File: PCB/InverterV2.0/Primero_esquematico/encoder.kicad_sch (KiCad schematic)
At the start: 25 parts, among them J5 348250125, U31 TPD4E05U06DQA, U32 TPD4E05U06DQA, U35 SN65HVD82DR, U36 AM26LS32AIDR, U37 SN74LVC245ANSR, U38 TPD4E05U06DQA

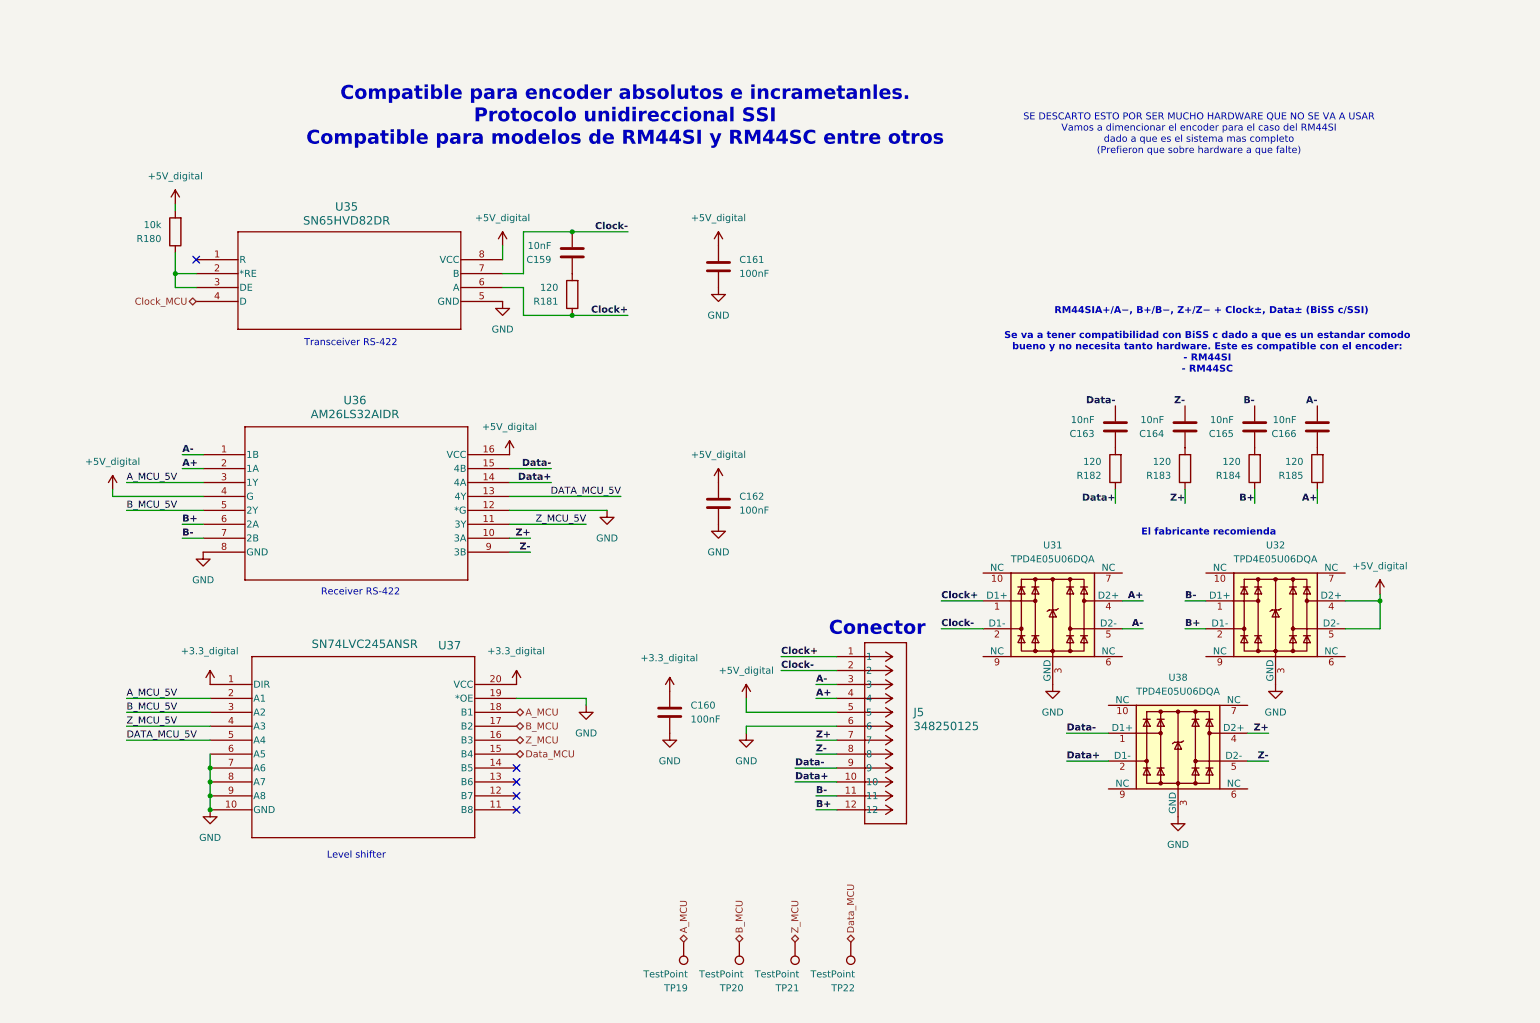
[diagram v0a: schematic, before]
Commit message: aislacion encoder
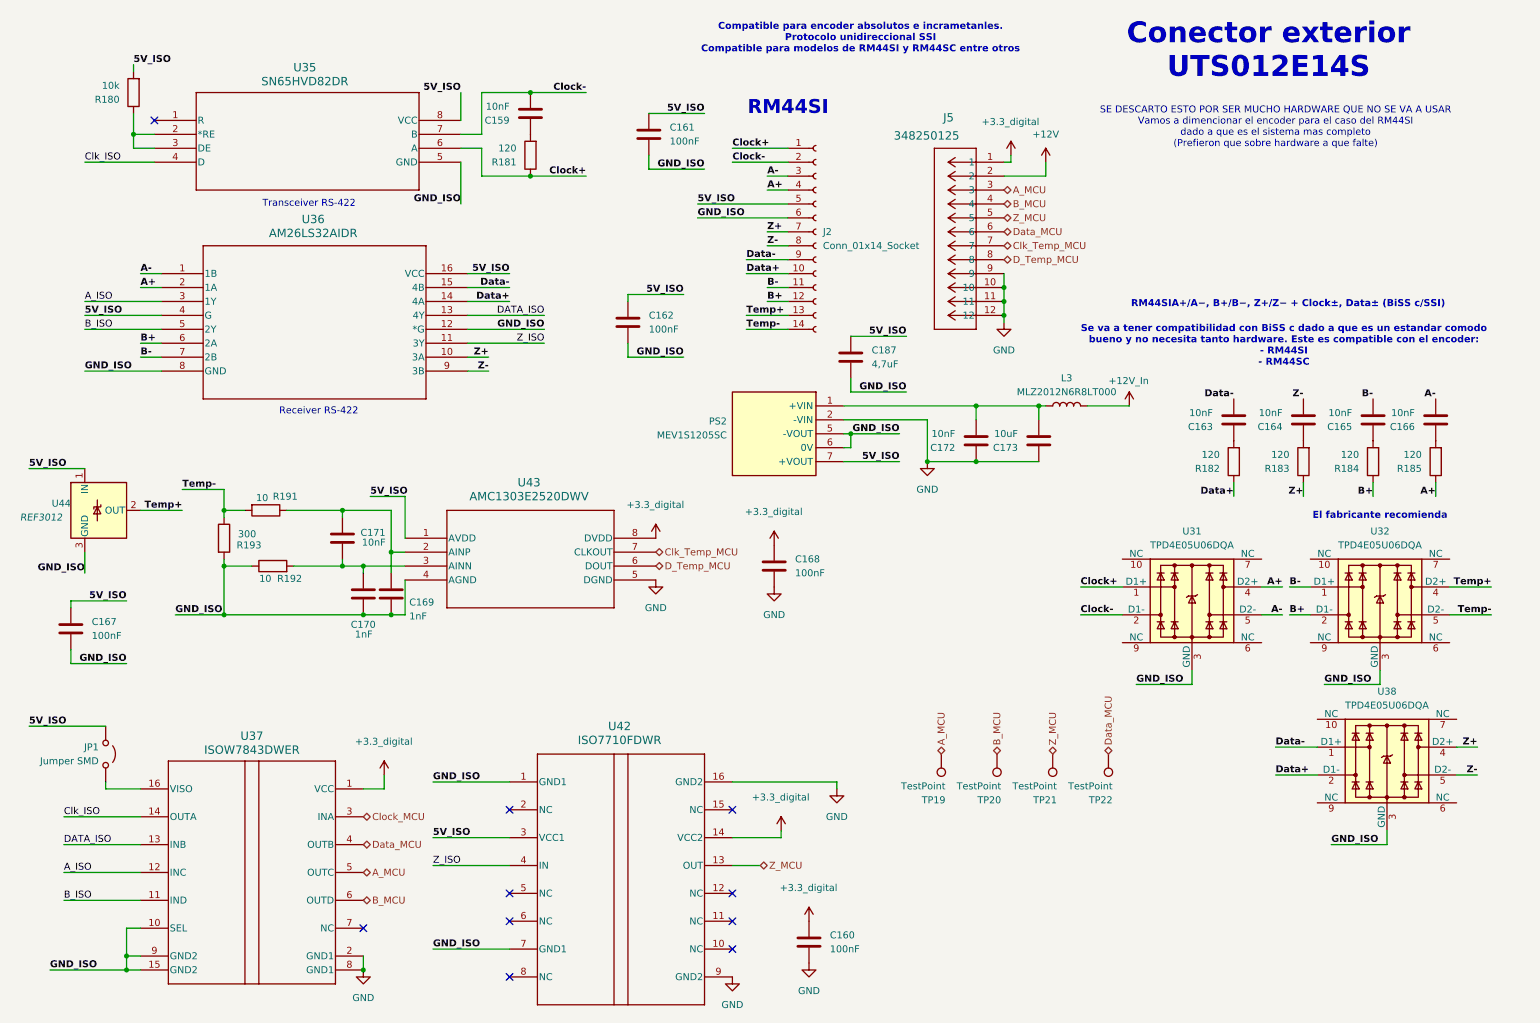
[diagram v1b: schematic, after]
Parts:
- removed U37: SN74LVC245ANSR, Snapeda:NS20-L, symbol Snapeda:SN74LVC245ANSR
- added C167, C168: 100nF, Capacitor_SMD:C_0603_1608Metric, symbol Device:C
- added C169, C170: 1nF, Capacitor_SMD:C_0603_1608Metric, symbol Device:C
- added C171, C172: 10nF, Capacitor_SMD:C_0603_1608Metric, symbol Device:C
- added C173: 10uF, Capacitor_SMD:C_0805_2012Metric, symbol Device:C
- added C187: 4,7uF, Capacitor_SMD:C_0805_2012Metric, symbol Device:C
- added J2: Conn_01x14_Socket, symbol Connector:Conn_01x14_Socket
- added JP1: Jumper SMD, symbol Jumper:Jumper_2_Open
- added L3: MLZ2012N6R8LT000, Inductor_SMD:L_0805_2012Metric, symbol Device:L
- added PS2: MEV1S1205SC, Snapeda:MEV1S1205SC, symbol Snapeda:MEV1S1205SC
- added R191, R192: 10, Resistor_SMD:R_0603_1608Metric, symbol Device:R
- added R193: 300, Resistor_SMD:R_0603_1608Metric, symbol Device:R
- added U37: ISOW7843DWER, Snapeda:DWE0016A, symbol Snapeda:ISOW7843DWER
- added U42: ISO7710FDWR, Snapeda:D0008B_HV, symbol Snapeda:ISO7710FDWR
- added U43: AMC1303E2520DWV, Snapeda:DWV0008A_TEX-L, symbol Snapeda:AMC1303E2520DWV
- added U44: REF3012, Package_TO_SOT_SMD:SOT-23, symbol Reference_Voltage:REF3012
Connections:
- net +3.3_digital: now also J5.1, C168.1, U37.1 (VCC), U42.14 (VCC2), U43.8 (DVDD)
- net A+: now also J2.4 (Pin_4); no longer J5.4
- net A-: now also J2.3 (Pin_3); no longer J5.3
- net A_MCU: now also J5.3, U37.5 (OUTC)
- net B+: now also J2.12 (Pin_12); no longer J5.12
- net B-: now also J2.11 (Pin_11); no longer J5.11
- net B_MCU: now also J5.4, U37.6 (OUTD)
- net Clock+: now also J2.1 (Pin_1); no longer J5.1
- net Clock-: now also J2.2 (Pin_2); no longer J5.2
- net Clock_MCU: now also U37.3 (INA); no longer U35.4 (D)
- net Data+: now also J2.10 (Pin_10); no longer J5.10
- net Data-: now also J2.9 (Pin_9); no longer J5.9
- net Data_MCU: now also J5.6, U37.4 (OUTB)
- net GND: now also J5.10, J5.11, J5.12, J5.9, C168.2, C172.2, C173.2, PS2.2 (-VIN), U37.2 (GND1), U37.8 (GND1), U42.16 (GND2), U42.9 (GND2), U43.5 (DGND); no longer C161.2, C162.2, J5.6, U31.3 (GND), U31.8 (GND), U32.3 (GND), U32.8 (GND), U35.5 (GND), U36.12 (*G), U36.8 (GND), U38.3 (GND), U38.8 (GND)
- net Z+: now also J2.7 (Pin_7); no longer J5.7
- net Z-: now also J2.8 (Pin_8); no longer J5.8
- net Z_MCU: now also J5.5, U42.13 (OUT)
- net +5V_digital renamed 5V_ISO
- net 5V_ISO: now also C167.1, C187.1, J2.5 (Pin_5), JP1.2 (B), PS2.7 (+VOUT), U42.3 (VCC1), U43.1 (AVDD), U44.1 (IN); no longer J5.5, U32.4 (D2+), U32.5 (D2-)
- net A_MCU_5V renamed A_ISO
- net A_ISO: now also U37.12 (INC)
- net B_MCU_5V renamed B_ISO
- net B_ISO: now also U37.11 (IND)
- net DATA_MCU_5V renamed DATA_ISO
- net DATA_ISO: now also U37.13 (INB)
- net Z_MCU_5V renamed Z_ISO
- net Z_ISO: now also U42.4 (IN)
- new net: JP1.1 (A), U37.16 (VISO)
- new net: C172.1, C173.1, L3.1, PS2.1 (+VIN)
- new net: C169.1, C171.1, R191.1, U43.2 (AINP)
- new net: C170.1, C171.2, R192.2, U43.3 (AINN)
- new net +12V: J5.2
- new net +12V_In: L3.2
- new net Clk_ISO: U35.4 (D), U37.14 (OUTA)
- new net Clk_Temp_MCU: J5.7, U43.7 (CLKOUT)
- new net D_Temp_MCU: J5.8, U43.6 (DOUT)
- new net GND_ISO: C161.2, C162.2, C167.2, C169.2, C170.2, C187.2, J2.6 (Pin_6), PS2.5 (-VOUT), PS2.6 (0V), R192.1, R193.2, U31.3 (GND), U31.8 (GND), U32.3 (GND), U32.8 (GND), U35.5 (GND), U36.12 (*G), U36.8 (GND), U37.10 (SEL), U37.15 (GND2), U37.9 (GND2), U38.3 (GND), U38.8 (GND), U42.1 (GND1), U42.7 (GND1), U43.4 (AGND), U44.3 (GND)
- new net Temp+: J2.13 (Pin_13), U32.4 (D2+), U44.2 (OUT)
- new net Temp-: J2.14 (Pin_14), R191.2, R193.1, U32.5 (D2-)
- no-connect marks 5 -> 10
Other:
- note added: "Conector exterior UTS012E14S"
- note added: "RM44SI"
- note removed: "Conector"
- note removed: "Level shifter"
- moved on the sheet: C159, C160, C161, C162, C163, C164, C165, C166, R180, R181, R182, R183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
